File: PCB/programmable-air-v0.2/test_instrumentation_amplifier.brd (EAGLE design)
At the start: 47.9 x 38.1 mm, 15 parts, among them IC1 INA126U, IC2 7805T

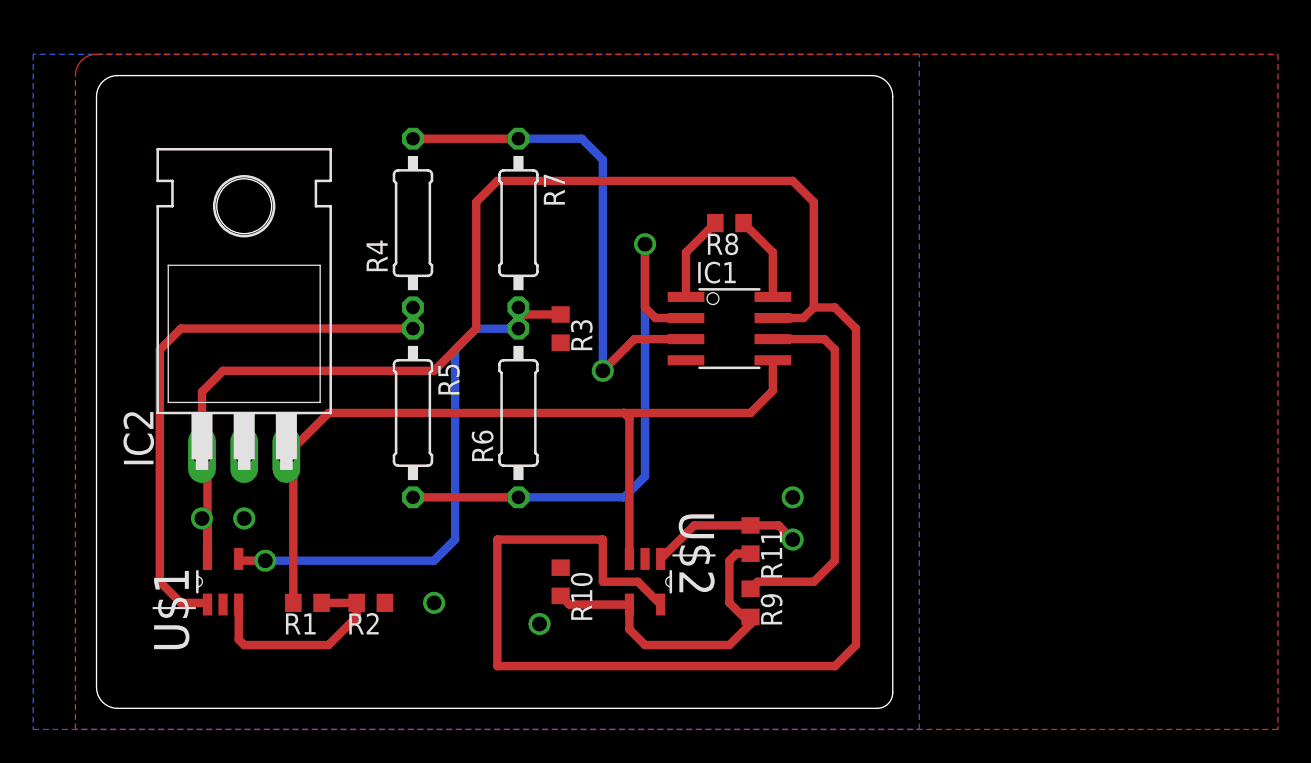
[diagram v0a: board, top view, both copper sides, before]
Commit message: LM358 test board ready
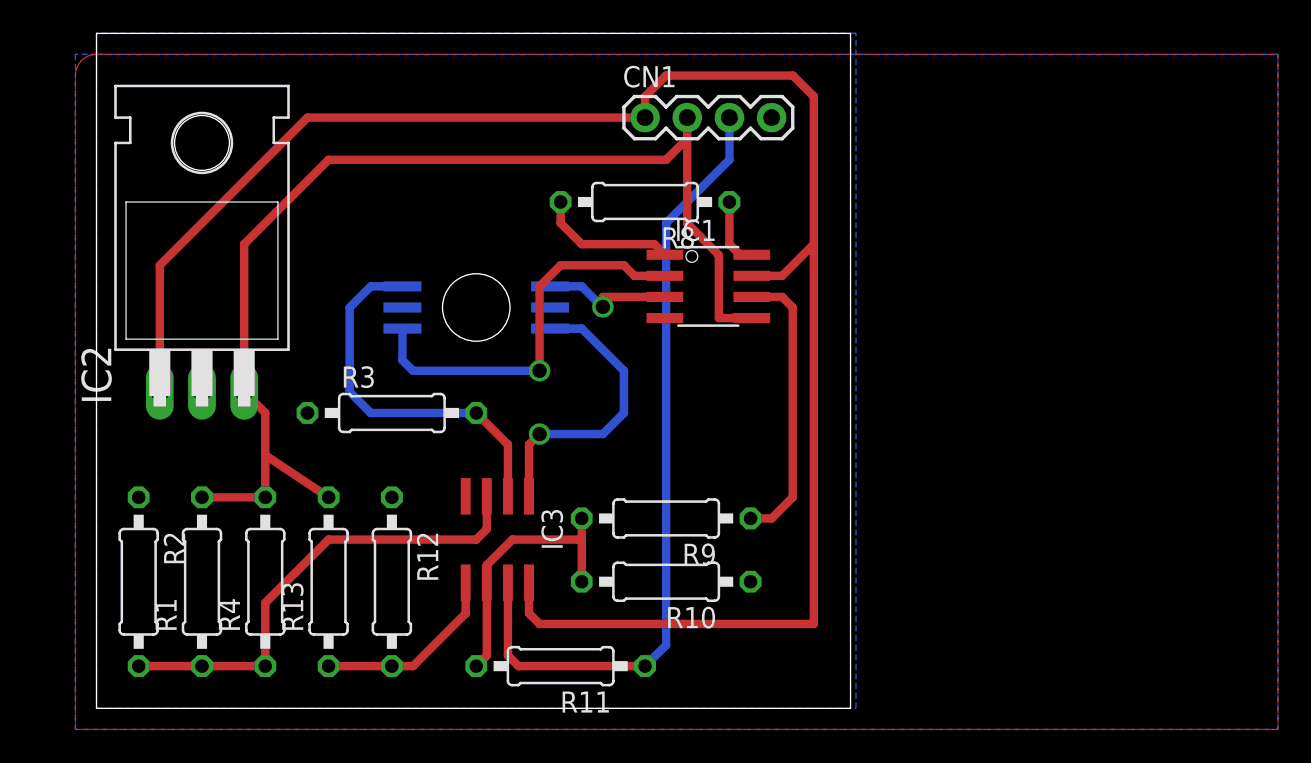
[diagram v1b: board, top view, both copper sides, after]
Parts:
- removed R5, R7: 20K, eagle-ltspice:0207/10
- removed R6: 19.9K, eagle-ltspice:0207/10
- removed U$2: MCP6001T-I/OT, MCP6001T-I_OT:SOT95P270X145-5N
- added CN1: 1X4-BIG, adafruit:1X04-BIG
- added IC3: LM358MX, linear:SO08
- added R12, R13: (no value), eagle-ltspice:0207/10
- R1, R10, R11, R2, R3, R8, R9: device eagle-ltspice:R0603 -> eagle-ltspice:0207/10
- R4: value 20K -> 15K
- U$1: value MCP6001T-I/OT -> 2SMPP-03; device MCP6001T-I_OT:SOT95P270X145-5N -> programmable-air-components:2SMPP-03
- moved R4 23.3 mm to (10.2, 7.62)
- moved U$1 22.5 mm to (22.9, 24.1), turned to 180 degrees
- moved R2 14.0 mm to (2.54, 7.62), turned to 270 degrees
- moved R11 13.7 mm to (27.9, 2.54), turned to 180 degrees
- moved R3 11.4 mm to (17.8, 17.8), turned to 0 degrees
- moved R9 7.18 mm to (34.3, 11.4), turned to 180 degrees
- moved R1 6.48 mm to (6.35, 7.62), turned to 90 degrees
- moved R10 6.35 mm to (34.3, 7.62), turned to 180 degrees
- moved R8 5.24 mm to (33.0, 30.5)
- moved IC2 4.58 mm to (6.35, 29.2)
- moved IC1 2.84 mm to (36.8, 25.4)
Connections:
- removed net N$6: R3.1, R6.2, R7.2, U$1.4
- new net N$11: IC3.5, R12.2, R13.1
- new net N$13: IC3.2, R3.2, U$1.P$3
- net GND: now also CN1.4, IC3.4, R12.1, R3.1; no longer R3.2, U$1.2, U$2.2
- net N$1: now also IC3.6; no longer U$2.4
- net N$10: now also IC3.3, R4.1; no longer U$1.3
- net N$12: now also CN1.3, IC3.7; no longer U$2.1
- net N$3: now also U$1.P$4; no longer R4.2, R7.1
- net N$4: now also CN1.2, R13.2, R4.2; no longer U$2.3
- net N$7: now also U$1.P$1; no longer R5.2, R6.1
- net N$8: now also IC3.1, U$1.P$6; no longer R4.1, R5.1, U$1.1
- net VCC: now also CN1.1, IC3.8; no longer U$1.5, U$2.5
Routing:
- net N$12: track 9.14 -> 48.0 mm, vias 1 -> 0
- net N$6: track 33.3 -> 0.00 mm, vias 1 -> 0
- net VCC: track 133.7 -> 108.5 mm, vias 1 -> 0
- net N$13: track 0.00 -> 22.7 mm
- net N$3: track 30.4 -> 8.05 mm
- net N$4: track 50.7 -> 68.3 mm
- net N$8: track 34.4 -> 17.7 mm, vias 0 -> 1
- net N$10: track 13.0 -> 28.6 mm
- net N$11: track 0.00 -> 11.4 mm
- net N$7: track 35.0 -> 23.8 mm
- net N$9: track 22.5 -> 17.2 mm
- net N$1: track 20.3 -> 16.5 mm
- net N$5: track 5.18 -> 8.33 mm
- net N$2: track 5.18 -> 4.15 mm
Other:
- board size 47.9 x 38.1 mm -> 45.4 x 40.6 mm
